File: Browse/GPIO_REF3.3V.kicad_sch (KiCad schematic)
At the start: 10 parts, among them IC3 TPS2121RUXT

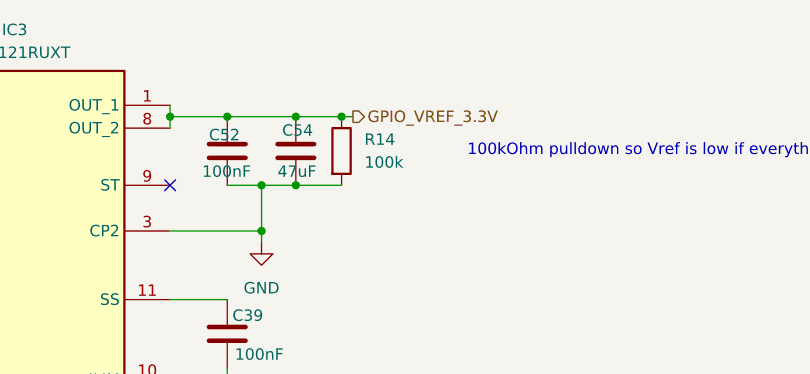
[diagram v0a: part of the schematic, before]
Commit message: Deploying to gh-pages from @ Nautilus-UUV/nautilus-mainboard-PCB@62d9beca31554f779583bfc3c938b3f82a581309 🚀
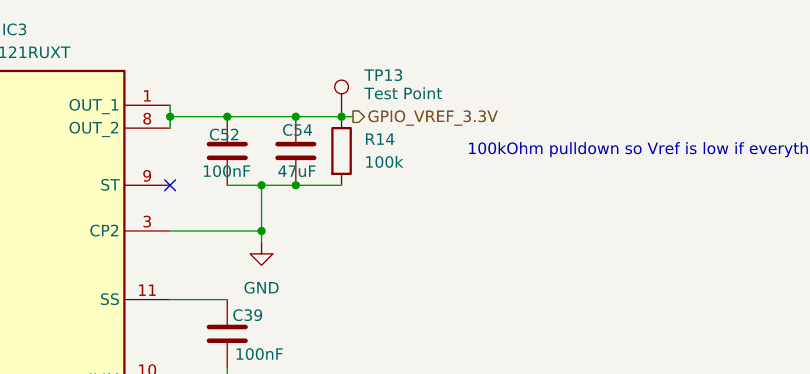
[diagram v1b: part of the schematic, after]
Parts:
- added TP13: Test Point, TestPoint:TestPoint_Pad_D1.5mm, symbol #dzdb:g_mech/M-TEST-SMT_1.5mm_round
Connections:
- net GPIO_VREF_3.3V: now also TP13.1
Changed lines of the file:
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@@
+    )
+  )
+  (symbol (lib_id "#dzdb:g_mech/M-TEST-SMT_1.5mm_round") (at 172.72 77.47 0) (unit 1)
+    (exclude_from_sim no) (in_bom yes) (on_board yes) (dnp no)
+    (property "Reference" "TP13" (at 175.26 72.8979 0)
+      (effects (font (size 1.27 1.27)) (justify left))
+    )
+    (property "Value" "Test Point" (at 175.26 74.93 0)
+      (effects (font (size 1.27 1.27)) (justify left))
+    )
+    (property "Footprint" "TestPoint:TestPoint_Pad_D1.5mm" (at 177.8 77.47 0)
+      (effects (font (size 1.27 1.27)) (hide yes))
+    )
+    (property "Datasheet" "~" (at 177.8 77.47 0)
+      (effects (font (size 1.27 1.27)) (hide yes))
+    )
+    (property "Description" "SMT Test Point 1.5mm round" (at 172.72 77.47 0)
+      (effects (font (size 1.27 1.27)) (hide yes))
+    )
+    (property "IPN" "M-TEST-SMT_1.5mm_round" (at 172.72 77.47 0)
+      (effects (font (size 1.27 1.27)) (hide yes))
+    )
+    (property "Comments" "TestPoint 1.5mm" (at 172.72 77.47 0)
+      (effects (font (size 1.27 1.27)) (hide yes))
+    )
+    (pin "1")
+    (instances
+      (project "nautilus_mainboard"
+        (path "/ce1819b2-f280-40ed-834f-6fe4d12f809d/c1998c4d-3f9a-4761-b447-a813532738a0/b9b676f4-45ad-4d4b-96a9-894c1f9d02cb"
+          (reference "TP13") (unit 1)
+        )
+      )
     )
   )
